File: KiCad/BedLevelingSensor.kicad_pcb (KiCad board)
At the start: 2 copper layers, 12.2 x 17 mm, 9 parts, among them J1 CONN_01X02, J2 CONN_01X02, J3 CONN_01X03, U1 ATTINY15-1SC, U2 L9110

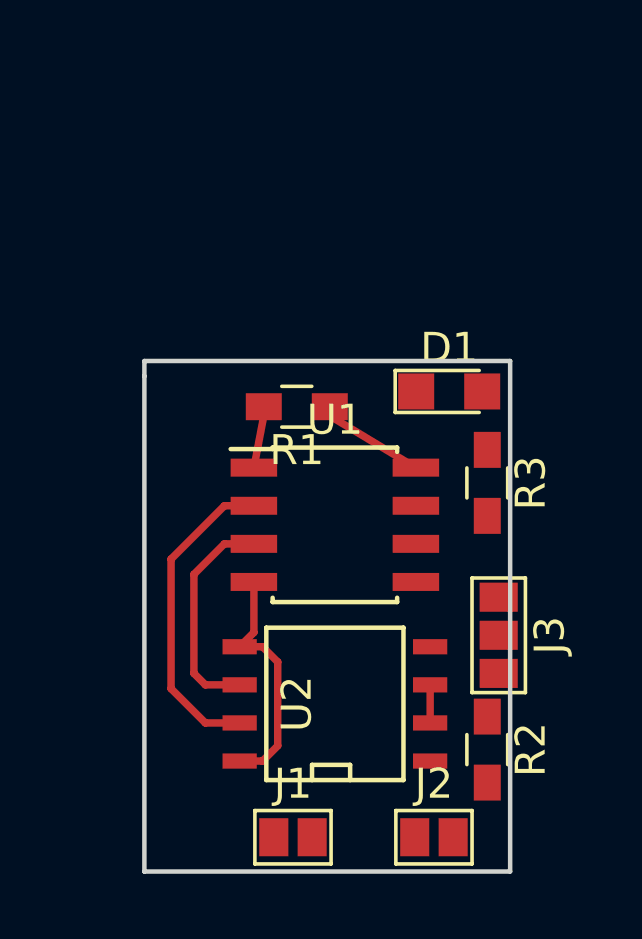
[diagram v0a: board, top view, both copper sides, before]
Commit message: Schematic and PCB
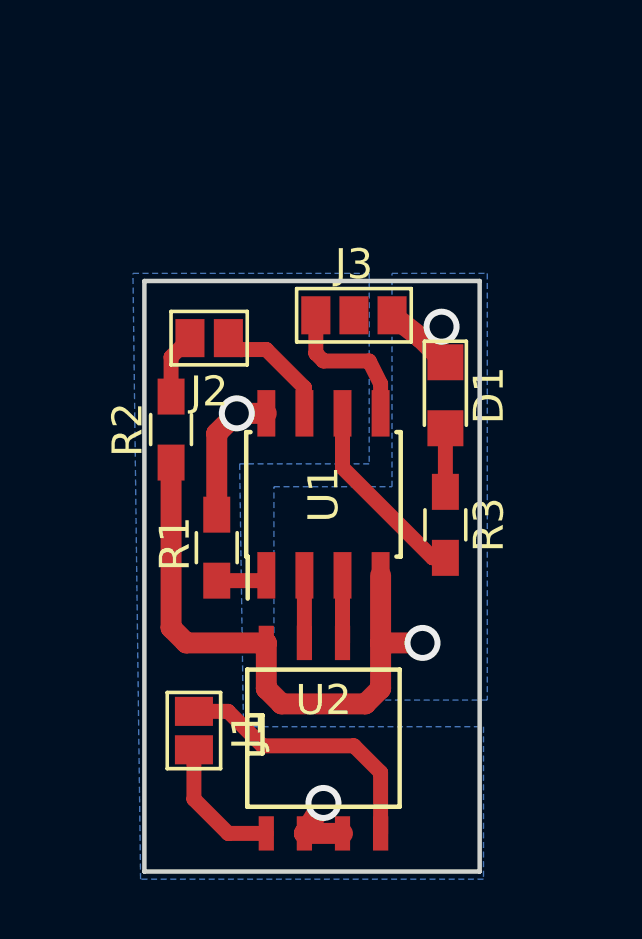
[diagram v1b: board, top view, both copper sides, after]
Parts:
- J1: value CONN_01X02 -> SOLENOID
- J2: value CONN_01X02 -> Sensor
- J3: value CONN_01X03 -> Input
- moved J2 18.2 mm to (134.2, 108.1), turned to 270 degrees
- moved R2 15.0 mm to (133.0, 111.1), turned to 90 degrees
- moved J3 11.7 mm to (139.1, 107.3), turned to 270 degrees
- moved R1 5.40 mm to (134.5, 115.1), turned to 270 degrees
- moved J1 4.85 mm to (133.7, 121.2), turned to 0 degrees
- moved R3 1.98 mm to (142.1, 114.3)
- moved U2 1.20 mm to (138.0, 121.4), turned to 0 degrees
- moved U1 1.09 mm to (138.0, 113.3), turned to 90 degrees
- moved D1 0.18 mm to (142.1, 110.0), turned to 270 degrees
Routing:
- net GND: track 8.11 -> 23.0 mm, vias 0 -> 2
- net Net-(J1-Pad1): track 0.00 -> 9.10 mm
- net IB: track 10.6 -> 2.25 mm
- net LED: track 0.00 -> 6.48 mm
- net IA: track 7.40 -> 2.25 mm
- net Net-(J3-Pad3): track 0.00 -> 4.99 mm
- net Net-(J1-Pad2): track 0.00 -> 4.53 mm
- net Net-(J2-Pad1): track 0.00 -> 4.07 mm
- net VCC: track 4.92 -> 7.46 mm, vias 0 -> 2
- net Net-(J2-Pad2): track 0.00 -> 2.21 mm
- net Net-(D1-Pad2): track 0.00 -> 2.12 mm
- added copper zone on B.Cu, net GND
- added copper zone on B.Cu, net VCC
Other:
- board size 12.2 x 17 mm -> 11.2 x 19.7 mm
- net class Default: trace_width 0.25 -> 0.5; via_dia 0.6 -> 1.2; via_drill 0.4 -> 0.8
- net class POWER added: clearance 0.2, trace_width 0.7, via_dia 1.2, via_drill 0.8

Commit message: Schematic/PCB adjust
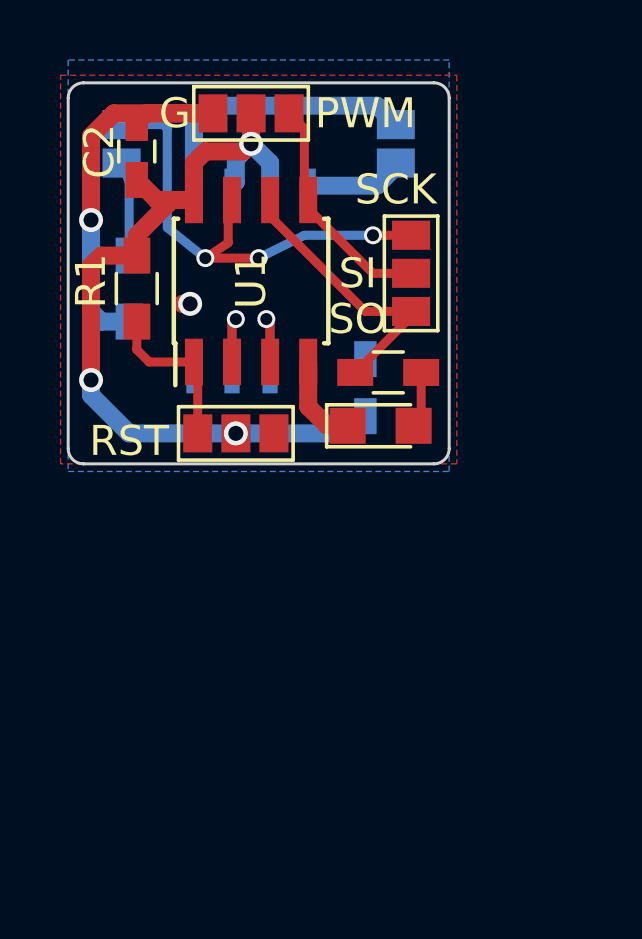
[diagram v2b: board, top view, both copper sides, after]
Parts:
- added C1: 2.2uf, Capacitors_SMD:C_0603_HandSoldering, B.Cu at (139.4, 109.7)
- added C2: 100n, Capacitors_SMD:C_0603_HandSoldering, F.Cu at (131.8, 101.9)
- added J4: Prog?dat, Connectors:GS3, F.Cu at (141.0, 105.9)
- added J5: Prog?pwr, Connectors:GS3, F.Cu at (135.1, 111.3)
- J1, J2, R2, U2: moved to B.Cu
- moved J1 20.7 mm to (140.5, 101.6)
- moved U2 15.4 mm to (135.6, 106.2)
- moved R1 9.04 mm to (131.8, 106.4)
- moved J3 7.55 mm to (135.6, 100.6), turned to 90 degrees
- moved U1 7.51 mm to (135.6, 106.2)
- moved J2 7.11 mm to (131.3, 101.6), turned to 180 degrees
- moved R3 5.43 mm to (140.2, 109.2), turned to 180 degrees
- moved R2 4.90 mm to (131.6, 106.4)
- moved D1 2.39 mm to (140.0, 111.0), turned to 0 degrees
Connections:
- net Net-(J2-Pad1) renamed SCK
- net Net-(J3-Pad3) renamed MOSI
- net Net-(R1-Pad2) renamed RST
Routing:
- net VCC: track 7.46 -> 28.9 mm, vias 2 -> 3
- net SCK: track 4.07 -> 15.9 mm, vias 0 -> 3
- net Net-(J1-Pad1): track 9.10 -> 3.31 mm
- net GND: track 23.0 -> 17.4 mm, vias 2 -> 1
- net Net-(J1-Pad2): track 4.53 -> 9.29 mm
- net RST: track 1.72 -> 5.44 mm
- net LED: track 6.48 -> 9.36 mm
- net MOSI: track 4.99 -> 7.76 mm
- net IB: track 2.25 -> 3.44 mm, vias 0 -> 1
- net IA: track 2.25 -> 3.44 mm, vias 0 -> 1
- net Net-(J2-Pad2): track 2.21 -> 3.14 mm
- net (no net): track 0.00 -> 0.51 mm, vias 0 -> 1
- added copper zone on F.Cu, net GND
- removed copper zone on B.Cu, net VCC
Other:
- board size 11.2 x 19.7 mm -> 12.7 x 12.7 mm
- net class Default: trace_width 0.5 -> 0.3; via_dia 1.2 -> 0.6; via_drill 0.8 -> 0.4
- net class POWER: trace_width 0.7 -> 0.6; via_dia 1.2 -> 0.8; via_drill 0.8 -> 0.5
- rule pad_to_mask_clearance: 0.2 -> 0
- board text added: "Coil"
- board text added: "G"
- board text added: "PWM"
- board text added: "RST"
- board text added: "SCK"
- board text added: "SI"
- board text added: "SO"
- board text added: "Sense"
